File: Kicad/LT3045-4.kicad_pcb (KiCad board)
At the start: 4 copper layers, 100 x 50 mm, 36 parts, among them J1 Conn_Coaxial_Power, J2 Conn_Coaxial_Power, U1 LT3042, U2 LT3042, U3 LT3042, U4 LT3042

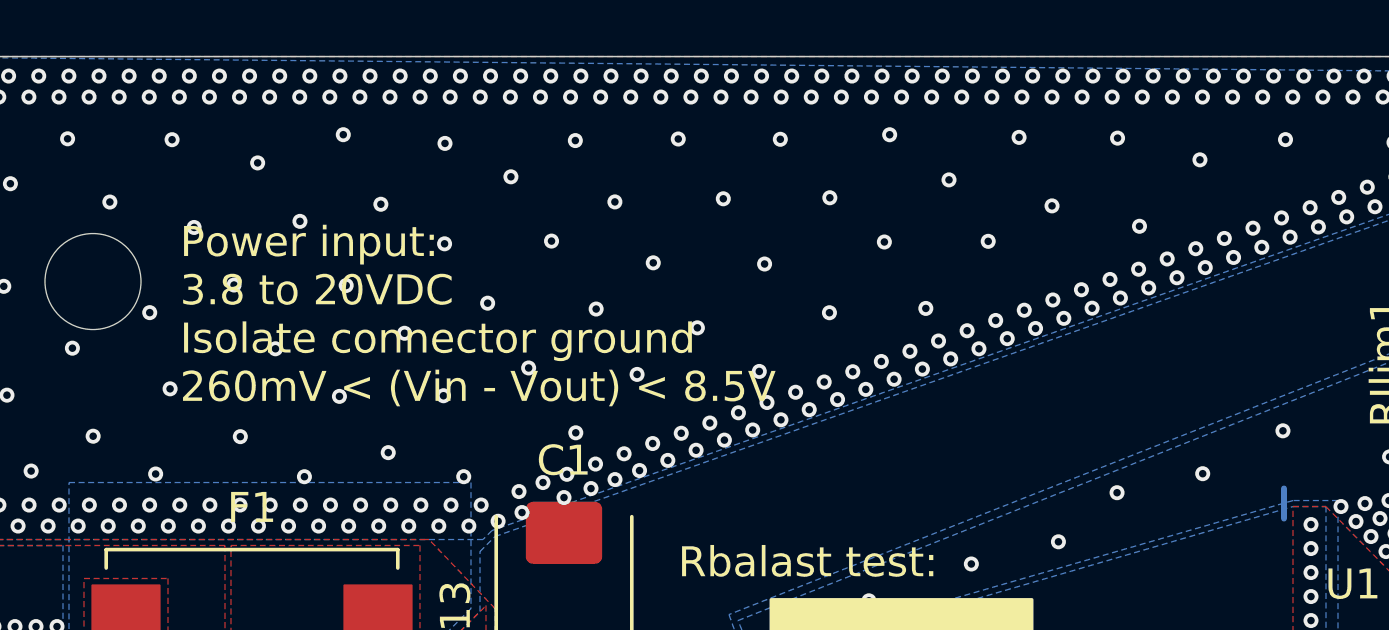
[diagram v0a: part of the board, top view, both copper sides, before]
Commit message: 1st LNA
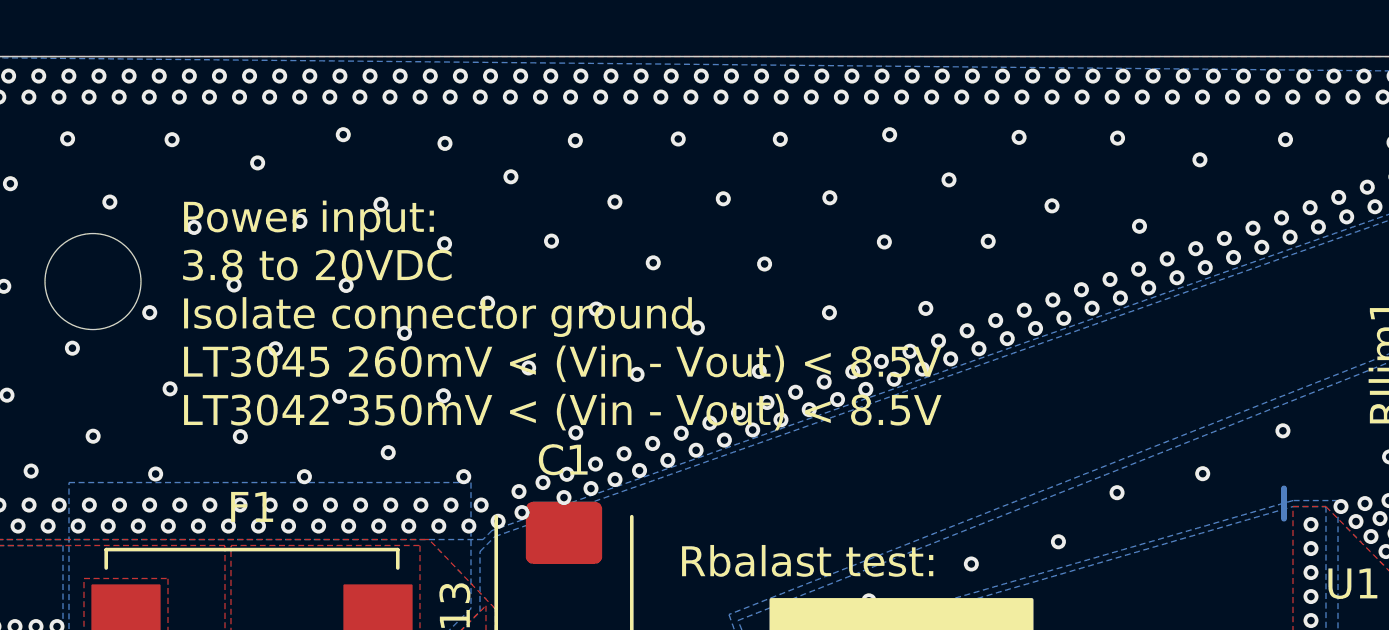
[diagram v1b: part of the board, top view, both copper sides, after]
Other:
- board text added: "Power input: 3.8 to 20VDC Isolate connector ground LT3045 260mV < (Vin - Vout) < 8.5V LT3042 350mV < (Vin - Vout) < 8.5V"
- board text removed: "Power input: 3.8 to 20VDC Isolate connector ground 260mV < (Vin - Vout) < 8.5V"
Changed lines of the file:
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@@
     (effects (font (size 1 1) (thickness 0.15)) (justify left))
   )
-  (gr_text "Power input:\n3.8 to 20VDC\nIsolate connector ground\n260mV < (Vin - Vout) < 8.5V" (at 10.4 8.6) (layer F.SilkS)
+  (gr_text "Power input:\n3.8 to 20VDC\nIsolate connector ground\nLT3045 260mV < (Vin - Vout) < 8.5V\nLT3042 350mV < (Vin - Vout) < 8.5V" (at 10.4 8.6) (layer F.SilkS)
     (effects (font (size 1 1) (thickness 0.15)) (justify left))
   )
